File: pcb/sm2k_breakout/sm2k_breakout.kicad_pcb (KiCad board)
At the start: 2 copper layers, 3 parts

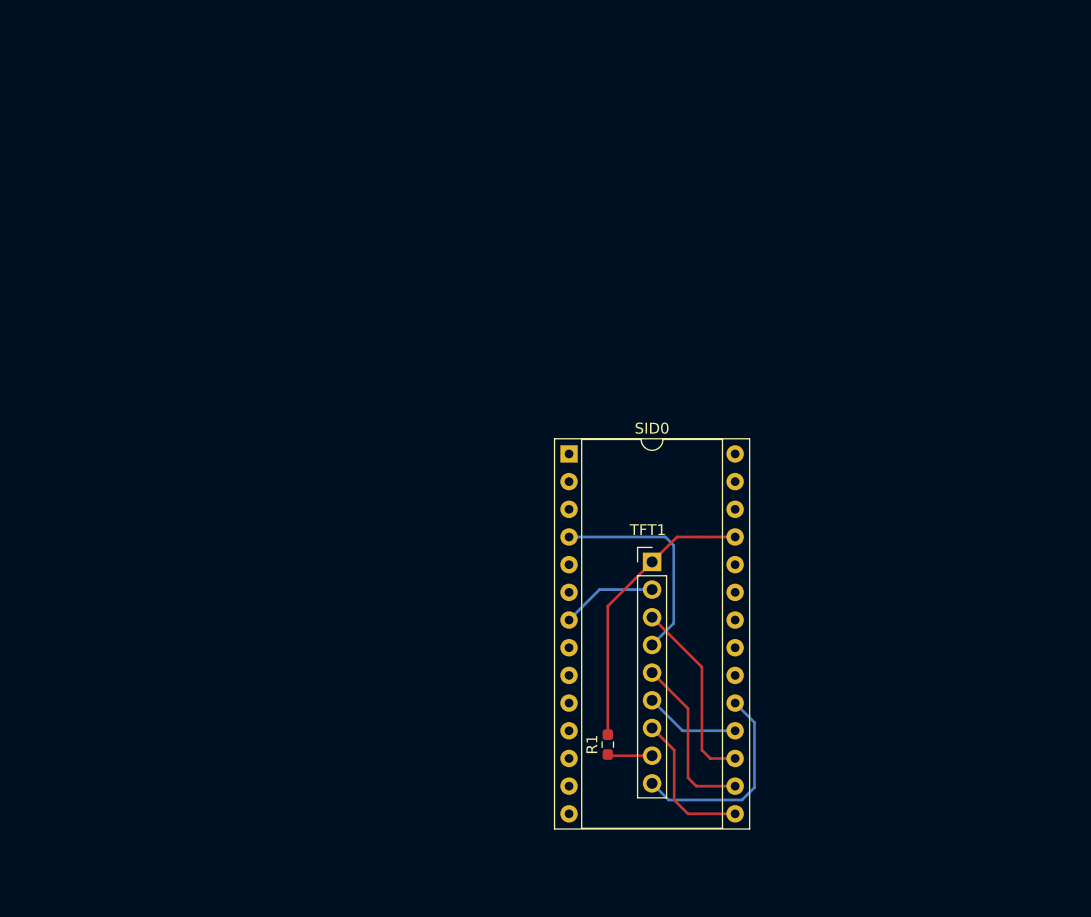
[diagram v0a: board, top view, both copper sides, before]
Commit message: button matrix
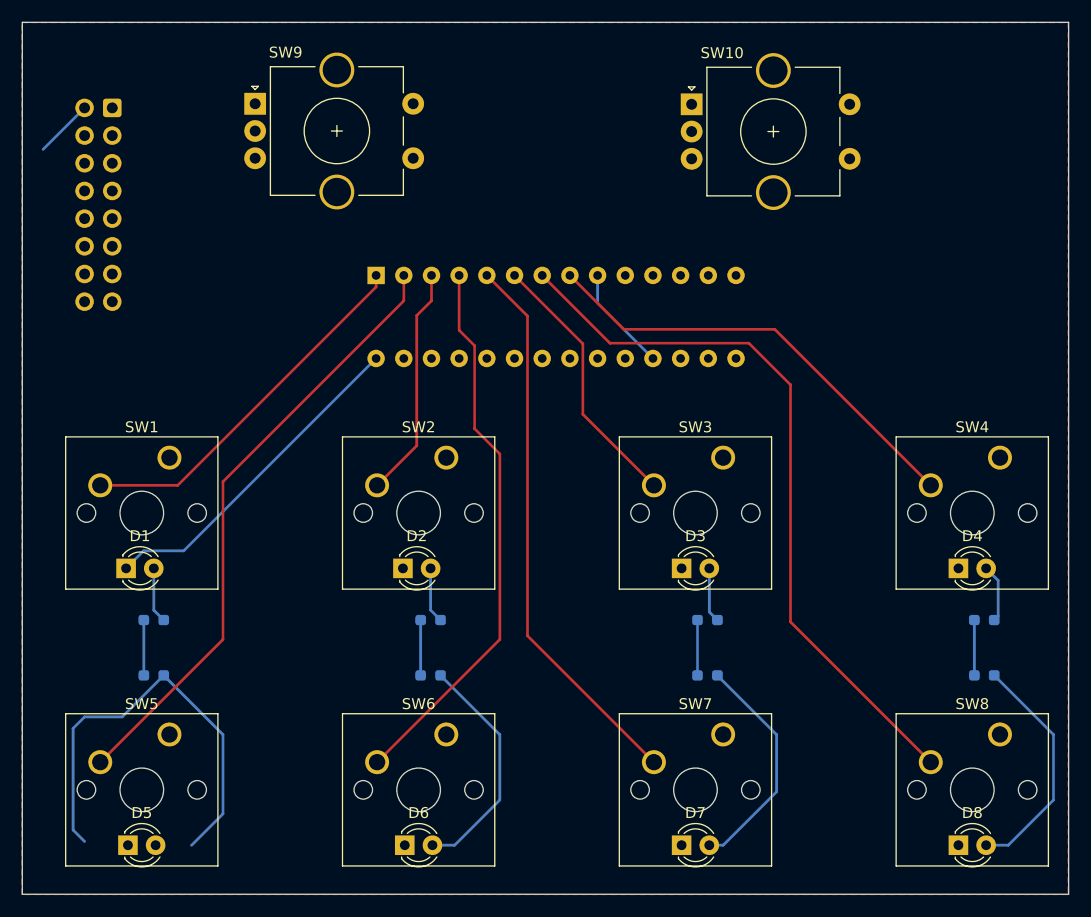
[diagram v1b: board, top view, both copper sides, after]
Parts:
- removed SID0: Conn_01x28, Package_DIP:DIP-28_W15.24mm_Socket
- removed TFT1: Conn_01x09, Connector_PinHeader_2.54mm:PinHeader_1x09_P2.54mm_Vertical
- added D1: LED, LED_THT:LED_D3.0mm, F.Cu at (162.6, 79.1)
- added D2: LED, LED_THT:LED_D3.0mm, F.Cu at (188.0, 79.1)
- added D3: LED, LED_THT:LED_D3.0mm, F.Cu at (213.5, 79.1)
- added D4: LED, LED_THT:LED_D3.0mm, F.Cu at (238.9, 79.1)
- added D5: LED, LED_THT:LED_D3.0mm, F.Cu at (162.7, 104.5)
- added D6: LED, LED_THT:LED_D3.0mm, F.Cu at (188.1, 104.5)
- added D7: LED, LED_THT:LED_D3.0mm, F.Cu at (213.5, 104.5)
- added D8: LED, LED_THT:LED_D3.0mm, F.Cu at (238.9, 104.5)
- added J1: Conn_01x16, Connector_IDC:IDC-Header_2x08_P2.54mm_Vertical, B.Cu at (161.3, 36.8)
- added R2: R_Small, Resistor_SMD:R_0603_1608Metric_Pad0.98x0.95mm_HandSolder, B.Cu at (190.5, 83.8)
- added R3: R_Small, Resistor_SMD:R_0603_1608Metric_Pad0.98x0.95mm_HandSolder, B.Cu at (215.9, 83.8)
- added R4: R_Small, Resistor_SMD:R_0603_1608Metric_Pad0.98x0.95mm_HandSolder, B.Cu at (241.3, 83.8)
- added R5: R_Small, Resistor_SMD:R_0603_1608Metric_Pad0.98x0.95mm_HandSolder, B.Cu at (165.1, 88.9)
- added R6: R_Small, Resistor_SMD:R_0603_1608Metric_Pad0.98x0.95mm_HandSolder, B.Cu at (190.5, 88.9)
- added R7: R_Small, Resistor_SMD:R_0603_1608Metric_Pad0.98x0.95mm_HandSolder, B.Cu at (215.9, 88.9)
- added R8: R_Small, Resistor_SMD:R_0603_1608Metric_Pad0.98x0.95mm_HandSolder, B.Cu at (241.3, 88.9)
- added SW1: SW_Push, Button_Switch_Keyboard:SW_Cherry_MX_1.00u_PCB, F.Cu at (166.5, 68.9)
- added SW10: RotaryEncoder_Switch, Rotary_Encoder:RotaryEncoder_Alps_EC11E-Switch_Vertical_H20mm_CircularMountingHoles, F.Cu at (214.4, 36.5)
- added SW2: SW_Push, Button_Switch_Keyboard:SW_Cherry_MX_1.00u_PCB, F.Cu at (191.9, 68.9)
- added SW3: SW_Push, Button_Switch_Keyboard:SW_Cherry_MX_1.00u_PCB, F.Cu at (217.3, 68.9)
- added SW4: SW_Push, Button_Switch_Keyboard:SW_Cherry_MX_1.00u_PCB, F.Cu at (242.7, 68.9)
- added SW5: SW_Push, Button_Switch_Keyboard:SW_Cherry_MX_1.00u_PCB, F.Cu at (166.5, 94.3)
- added SW6: SW_Push, Button_Switch_Keyboard:SW_Cherry_MX_1.00u_PCB, F.Cu at (191.9, 94.3)
- added SW7: SW_Push, Button_Switch_Keyboard:SW_Cherry_MX_1.00u_PCB, F.Cu at (217.3, 94.3)
- added SW8: SW_Push, Button_Switch_Keyboard:SW_Cherry_MX_1.00u_PCB, F.Cu at (242.7, 94.3)
- added SW9: RotaryEncoder_Switch, Rotary_Encoder:RotaryEncoder_Alps_EC11E-Switch_Vertical_H20mm_CircularMountingHoles, F.Cu at (174.4, 36.5)
- added U1: MCP23017_SP, Package_DIP:DIP-28_W7.62mm, B.Cu at (185.5, 52.2)
- R1: value 100 -> R_Small; moved to B.Cu
- moved R1 43.2 mm to (165.1, 83.8), turned to 0 degrees
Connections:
- R1 pad 1: TFT LED -> V3_3V
- R1 pad 2: V5V -> Net-(D1-Pad2)
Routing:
- net SW7: track 0.00 -> 66.9 mm
- net SW4: track 0.00 -> 56.2 mm
- net SW6: track 0.00 -> 51.0 mm
- net SW5: track 0.00 -> 50.9 mm
- net SW3: track 0.00 -> 41.1 mm
- net Net-(D5-Pad2): track 0.00 -> 40.2 mm
- net V3_3V: track 0.00 -> 35.4 mm
- net SW0: track 0.00 -> 33.9 mm
- net LED0: track 0.00 -> 30.9 mm
- net V5V: track 26.1 -> 0.00 mm
- net SW2: track 0.00 -> 24.6 mm
- net Net-(D8-Pad2): track 0.00 -> 21.6 mm
- net Net-(D6-Pad2): track 0.00 -> 21.6 mm
- net SW1: track 0.00 -> 21.3 mm
- net Net-(D7-Pad2): track 0.00 -> 21.1 mm
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- added copper zone on F.Cu, net GND
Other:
- board outline added: 96 x 80 mm
